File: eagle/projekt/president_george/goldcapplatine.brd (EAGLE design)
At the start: 32 x 36 mm, 5 parts

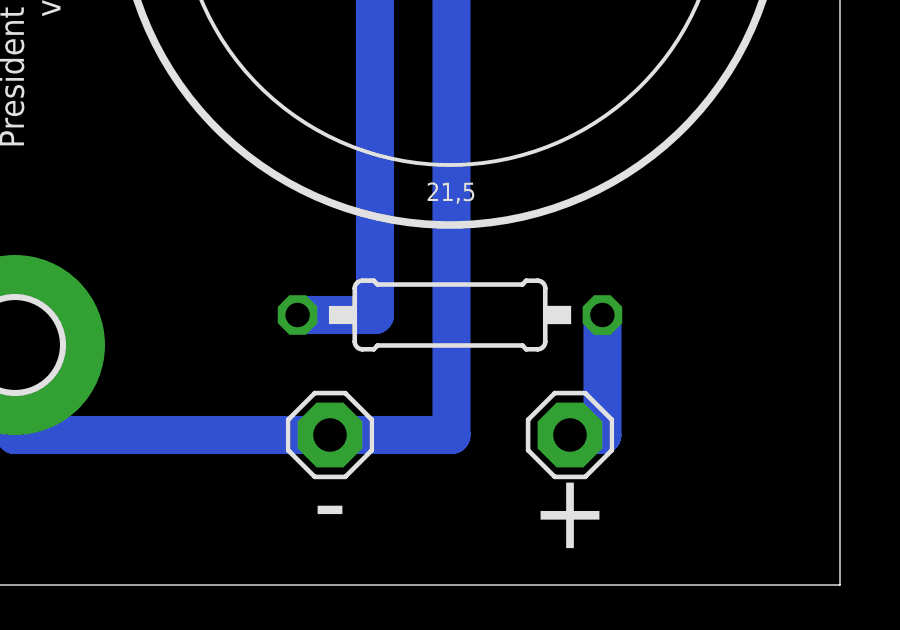
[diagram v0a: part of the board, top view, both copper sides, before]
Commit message: - checking the brd files
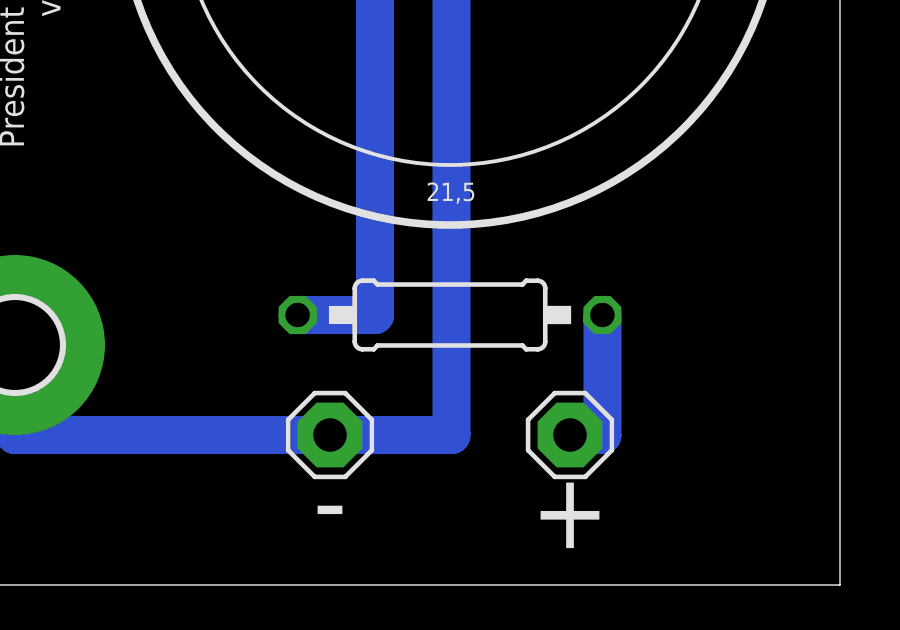
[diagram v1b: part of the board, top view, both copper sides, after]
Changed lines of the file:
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@@
 <layers>
 <layer number="1" name="Top" color="4" fill="1" visible="yes" active="yes"/>
-<layer number="2" name="Route2" color="1" fill="3" visible="no" active="no"/>
-<layer number="3" name="Route3" color="4" fill="3" visible="no" active="no"/>
-<layer number="4" name="Route4" color="1" fill="4" visible="no" active="no"/>
-<layer number="5" name="Route5" color="4" fill="4" visible="no" active="no"/>
-<layer number="6" name="Route6" color="1" fill="8" visible="no" active="no"/>
-<layer number="7" name="Route7" color="4" fill="8" visible="no" active="no"/>
+<layer number="2" name="Route2" color="1" fill="3" visible="no" active="yes"/>
+<layer number="3" name="Route3" color="4" fill="3" visible="no" active="yes"/>
+<layer number="4" name="Route4" color="1" fill="4" visible="no" active="yes"/>
+<layer number="5" name="Route5" color="4" fill="4" visible="no" active="yes"/>
+<layer number="6" name="Route6" color="1" fill="8" visible="no" active="yes"/>
+<layer number="7" name="Route7" color="4" fill="8" visible="no" active="yes"/>
 <layer number="8" name="Route8" color="1" fill="2" visible="no" active="no"/>
 <layer number="9" name="Route9" color="4" fill="2" visible="no" active="no"/>
@@
 </class>
 </classes>
-<designrules name="default">
-<description language="de">&lt;b&gt;EAGLE Design Rules&lt;/b&gt;
+<designrules name="Eagle_WEdirekt_150_check">
+<description language="de">
+WE &gt;/= 125µm Strukturen
+&lt;b&gt;EAGLE Design-Regeln&lt;/b&gt;
 &lt;p&gt;
-Die Standard-Design-Rules sind so gewählt, dass sie für
-die meisten Anwendungen passen. Sollte ihre Platine
-besondere Anforderungen haben, treffen Sie die erforderlichen
-Einstellungen hier und speichern die Design Rules unter
-einem neuen Namen ab.</description>
-<description language="en">&lt;b&gt;EAGLE Design Rules&lt;/b&gt;
-&lt;p&gt;
-The default Design Rules have been set to cover
-a wide range of applications. Your particular design
-may have different requirements, so please make the
-necessary adjustments and save your customized
-design rules under a new name.</description>
-<param name="layerSetup" value="(1*16)"/>
+Bitte nur von autorisierten erfahrenen Nutzern anwenden!!!
+</description>
+<param name="layerSetup" value="(1*2+3*4+5*6+7*16)"/>
 <param name="mtCopper" value="0.035mm 0.035mm 0.035mm 0.035mm 0.035mm 0.035mm 0.035mm 0.035mm 0.035mm 0.035mm 0.035mm 0.035mm 0.035mm 0.035mm 0.035mm 0.035mm"/>
-<param name="mtIsolate" value="1.5mm 0.15mm 0.2mm 0.15mm 0.2mm 0.15mm 0.2mm 0.15mm 0.2mm 0.15mm 0.2mm 0.15mm 0.2mm 0.15mm 0.2mm"/>
-<param name="mdWireWire" value="8mil"/>
-<param name="mdWirePad" value="8mil"/>
-<param name="mdWireVia" value="8mil"/>
+<param name="mtIsolate" value="0.2mm 0.15mm 0.2mm 0.15mm 0.2mm 0.15mm 0.2mm 0.15mm 0.2mm 0.15mm 0.2mm 0.15mm 0.2mm 0.15mm 0.2mm"/>
+<param name="mdWireWire" value="6mil"/>
+<param name="mdWirePad" value="6mil"/>
+<param name="mdWireVia" value="6mil"/>
 <param name="mdPadPad" value="8mil"/>
-<param name="mdPadVia" value="8mil"/>
-<param name="mdViaVia" value="8mil"/>
+<param name="mdPadVia" value="6mil"/>
+<param name="mdViaVia" value="6mil"/>
 <param name="mdSmdPad" value="8mil"/>
-<param name="mdSmdVia" value="8mil"/>
+<param name="mdSmdVia" value="6mil"/>
 <param name="mdSmdSmd" value="8mil"/>
 <param name="mdViaViaSameLayer" value="8mil"/>
 <param name="mnLayersViaInSmd" value="2"/>
-<param name="mdCopperDimension" value="40mil"/>
-<param name="mdDrill" value="8mil"/>
+<param name="mdCopperDimension" value="12mil"/>
+<param name="mdDrill" value="24mil"/>
 <param name="mdSmdStop" value="0mil"/>
-<param name="msWidth" value="10mil"/>
-<param name="msDrill" value="24mil"/>
+<param name="msWidth" value="6mil"/>
+<param name="msDrill" value="0.2mm"/>
 <param name="msMicroVia" value="9.99mm"/>
 <param name="msBlindViaRatio" value="0.5"/>
@@
 <param name="rvMicroViaOuter" value="0.25"/>
 <param name="rvMicroViaInner" value="0.25"/>
-<param name="rlMinPadTop" value="10mil"/>
+<param name="rlMinPadTop" value="9mil"/>
 <param name="rlMaxPadTop" value="20mil"/>
-<param name="rlMinPadInner" value="10mil"/>
+<param name="rlMinPadInner" value="9mil"/>
 <param name="rlMaxPadInner" value="20mil"/>
-<param name="rlMinPadBottom" value="10mil"/>
+<param name="rlMinPadBottom" value="9mil"/>
 <param name="rlMaxPadBottom" value="20mil"/>
-<param name="rlMinViaOuter" value="8mil"/>
-<param name="rlMaxViaOuter" value="20mil"/>
-<param name="rlMinViaInner" value="8mil"/>
-<param name="rlMaxViaInner" value="20mil"/>
-<param name="rlMinMicroViaOuter" value="4mil"/>
-<param name="rlMaxMicroViaOuter" value="20mil"/>
-<param name="rlMinMicroViaInner" value="4mil"/>
-<param name="rlMaxMicroViaInner" value="20mil"/>
+<param name="rlMinViaOuter" value="9mil"/>
+<param name="rlMaxViaOuter" value="12mil"/>
+<param name="rlMinViaInner" value="9mil"/>
+<param name="rlMaxViaInner" value="12mil"/>
+<param name="rlMinMicroViaOuter" value="6mil"/>
+<param name="rlMaxMicroViaOuter" value="8mil"/>
+<param name="rlMinMicroViaInner" value="6mil"/>
+<param name="rlMaxMicroViaInner" value="8mil"/>
 <param name="psTop" value="-1"/>
 <param name="psBottom" value="-1"/>
@@
 <param name="mvStopFrame" value="1"/>
 <param name="mvCreamFrame" value="0"/>
-<param name="mlMinStopFrame" value="4mil"/>
+<param name="mlMinStopFrame" value="3mil"/>
 <param name="mlMaxStopFrame" value="4mil"/>
 <param name="mlMinCreamFrame" value="0mil"/>
@@
 <param name="srMinRoundness" value="0mil"/>
 <param name="srMaxRoundness" value="0mil"/>
-<param name="slThermalIsolate" value="10mil"/>
+<param name="slThermalIsolate" value="12mil"/>
 <param name="slThermalsForVias" value="0"/>
 <param name="dpMaxLengthDifference" value="10mm"/>
@@
 <param name="checkFont" value="1"/>
 <param name="checkRestrict" value="1"/>
-<param name="useDiameter" value="13"/>
-<param name="maxErrors" value="50"/>
+<param name="useDiameter" value="31"/>
+<param name="maxErrors" value="999999"/>
 </designrules>
 <autorouter>
